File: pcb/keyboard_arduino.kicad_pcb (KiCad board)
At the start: 2 copper layers, 58.4 x 22.5 mm, 2 parts

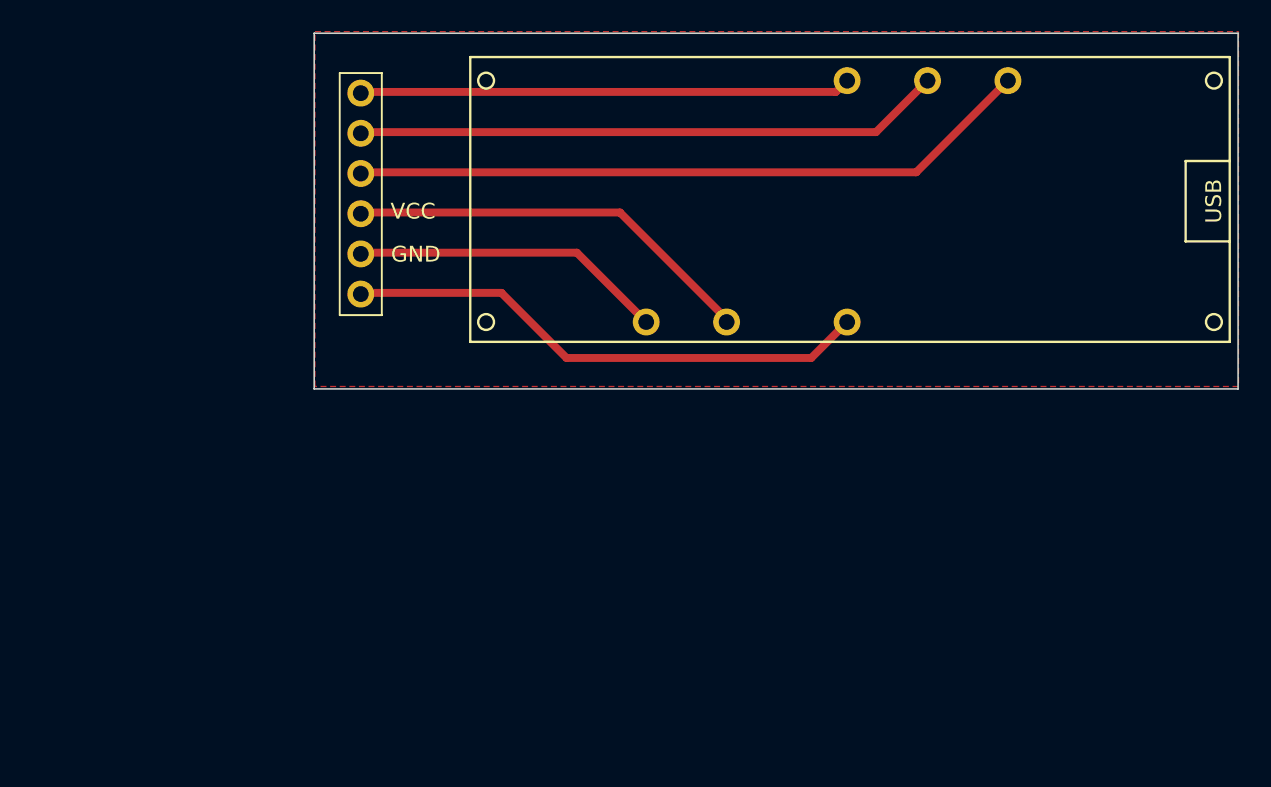
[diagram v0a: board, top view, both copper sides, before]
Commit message: Update pcb design
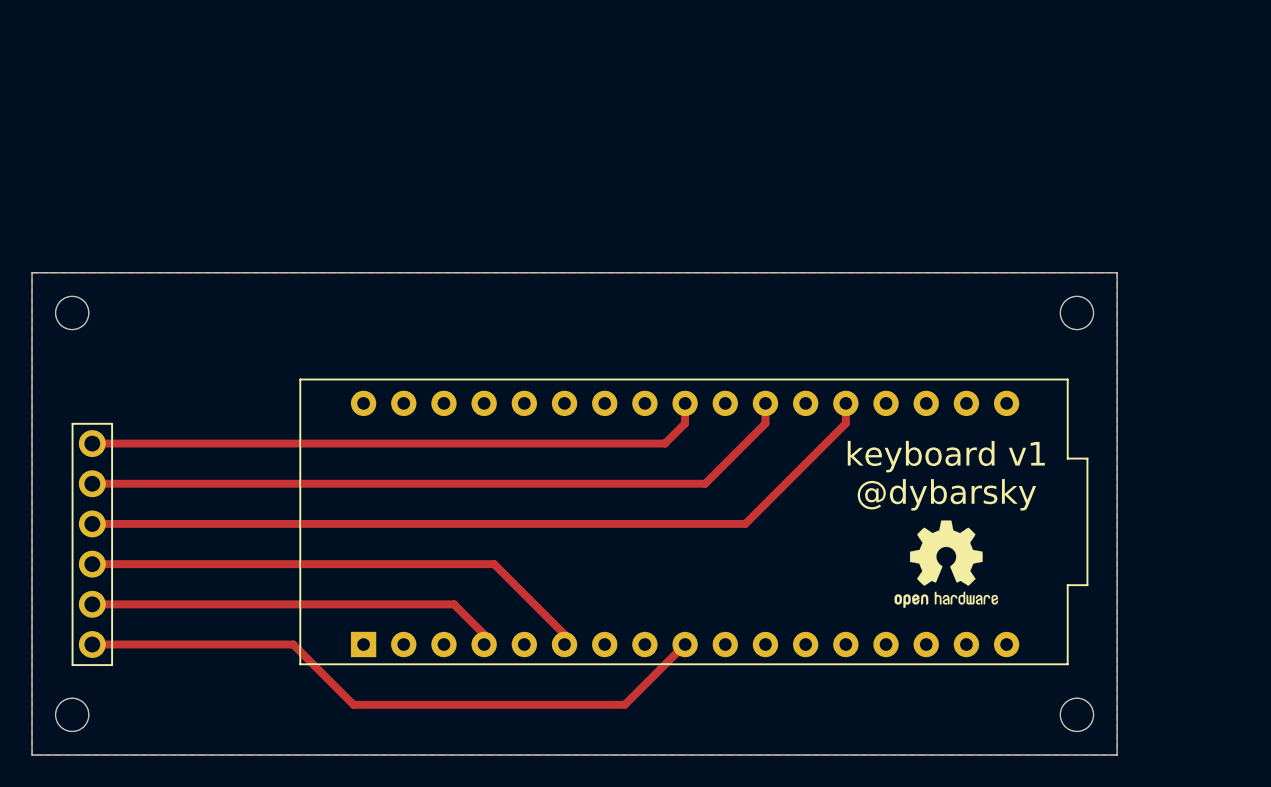
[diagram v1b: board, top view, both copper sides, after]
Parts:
- removed ARDUINO_MICRO_SHIELD: VAL**, arduino_micro:arduino_micro
- added REF**: OSHW-Logo2_7.3x6mm_SilkScreen, Symbol:OSHW-Logo2_7.3x6mm_SilkScreen, F.Cu at (98.4, 66.7)
- added REF**: MountingHole_2.1mm, MountingHole:MountingHole_2.1mm, F.Cu at (106.7, 50.8)
- added REF**: MountingHole_2.1mm, MountingHole:MountingHole_2.1mm, F.Cu at (43.2, 76.2)
- added REF**: Arduino_Micro, Arduino2:Arduino_Micro, F.Cu at (61.6, 71.8)
- added REF**: MountingHole_2.1mm, MountingHole:MountingHole_2.1mm, F.Cu at (43.2, 50.8)
- added REF**: MountingHole_2.1mm, MountingHole:MountingHole_2.1mm, F.Cu at (106.7, 76.2)
- moved REF** 27.9 mm to (44.5, 59.1)
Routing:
- net (no net): track 190.4 -> 235.3 mm
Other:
- board size 58.4 x 22.5 mm -> 68.6 x 30.5 mm
- board text added: "A5"
- board text added: "D4"
- board text added: "D6"
- board text added: "D8"
- board text added: "arduino micro"
- board text added: "keyboard v1 @dybarsky"
